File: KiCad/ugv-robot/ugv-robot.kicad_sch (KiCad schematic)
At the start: 2 parts, among them U1 Step Down DC DC

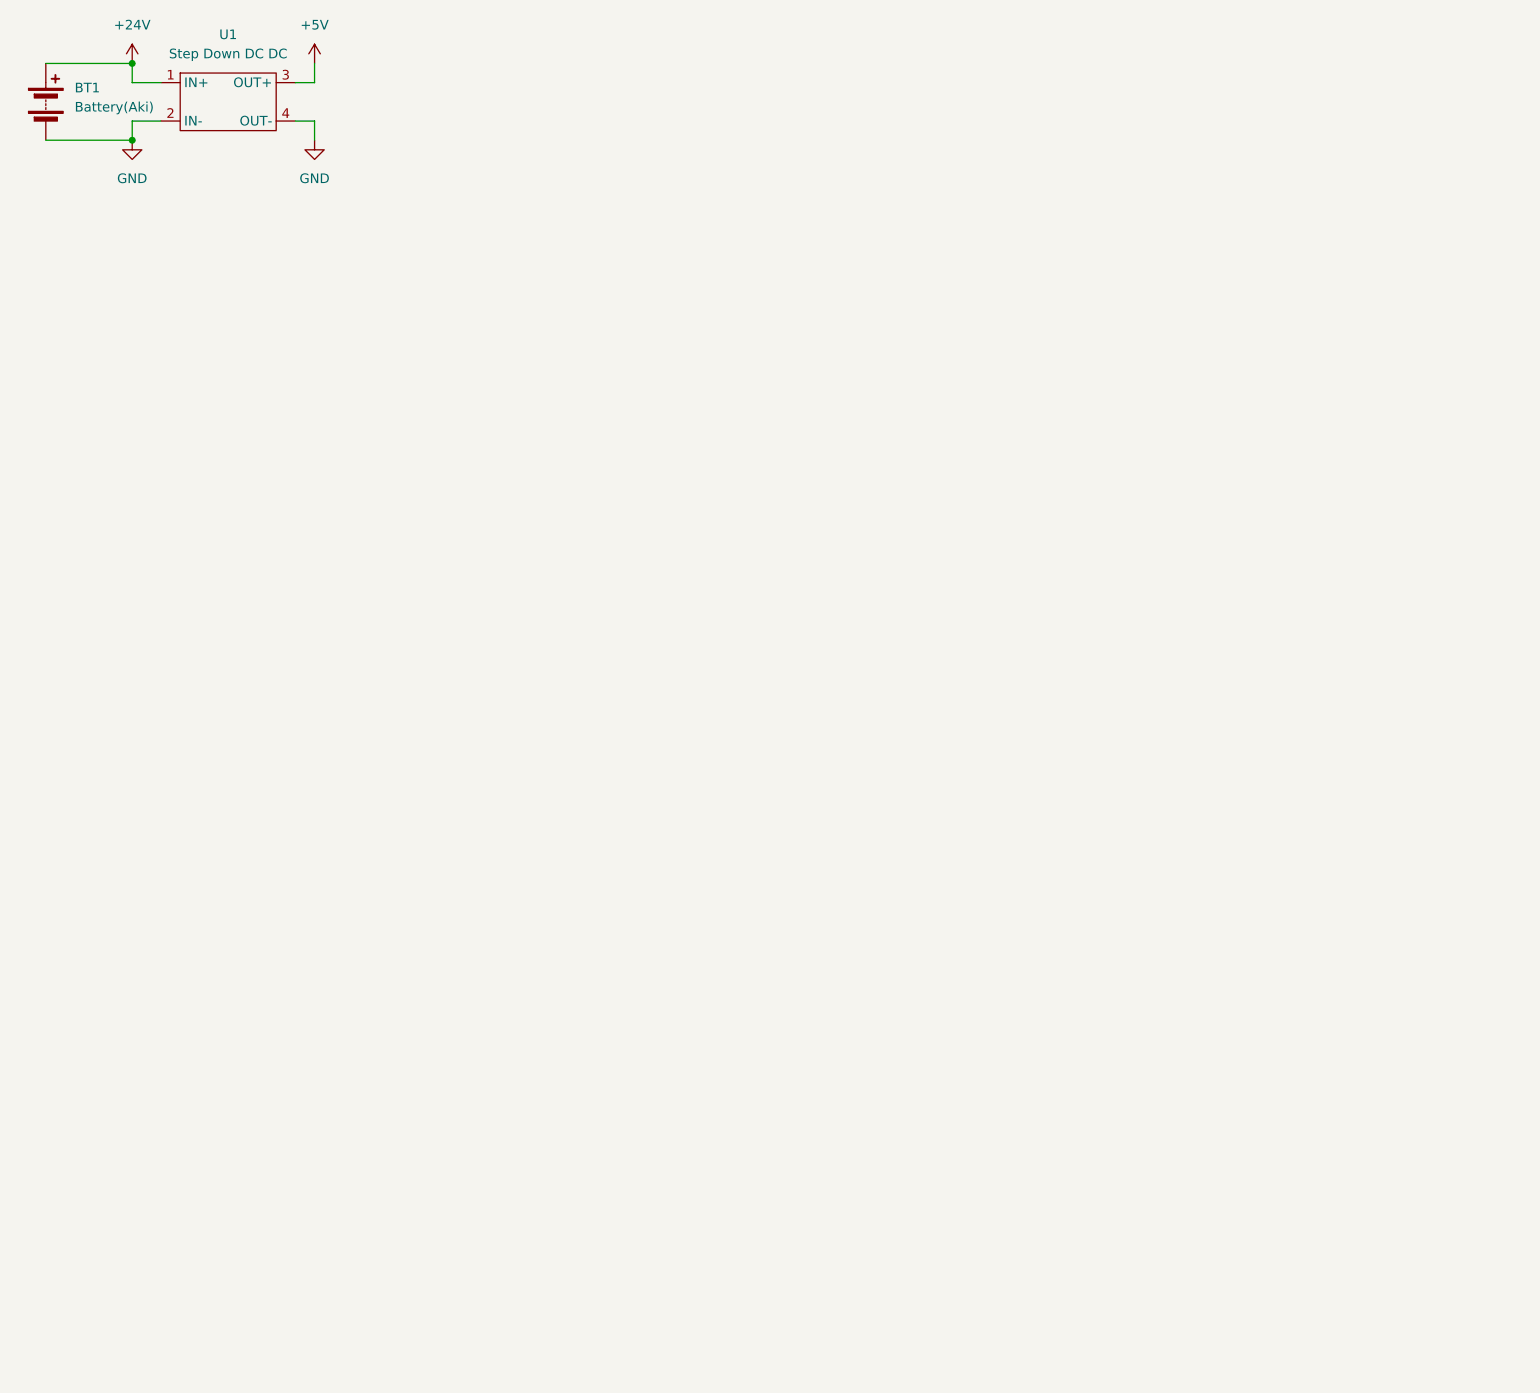
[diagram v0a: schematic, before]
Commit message: KiCad GCS (belum selesai)
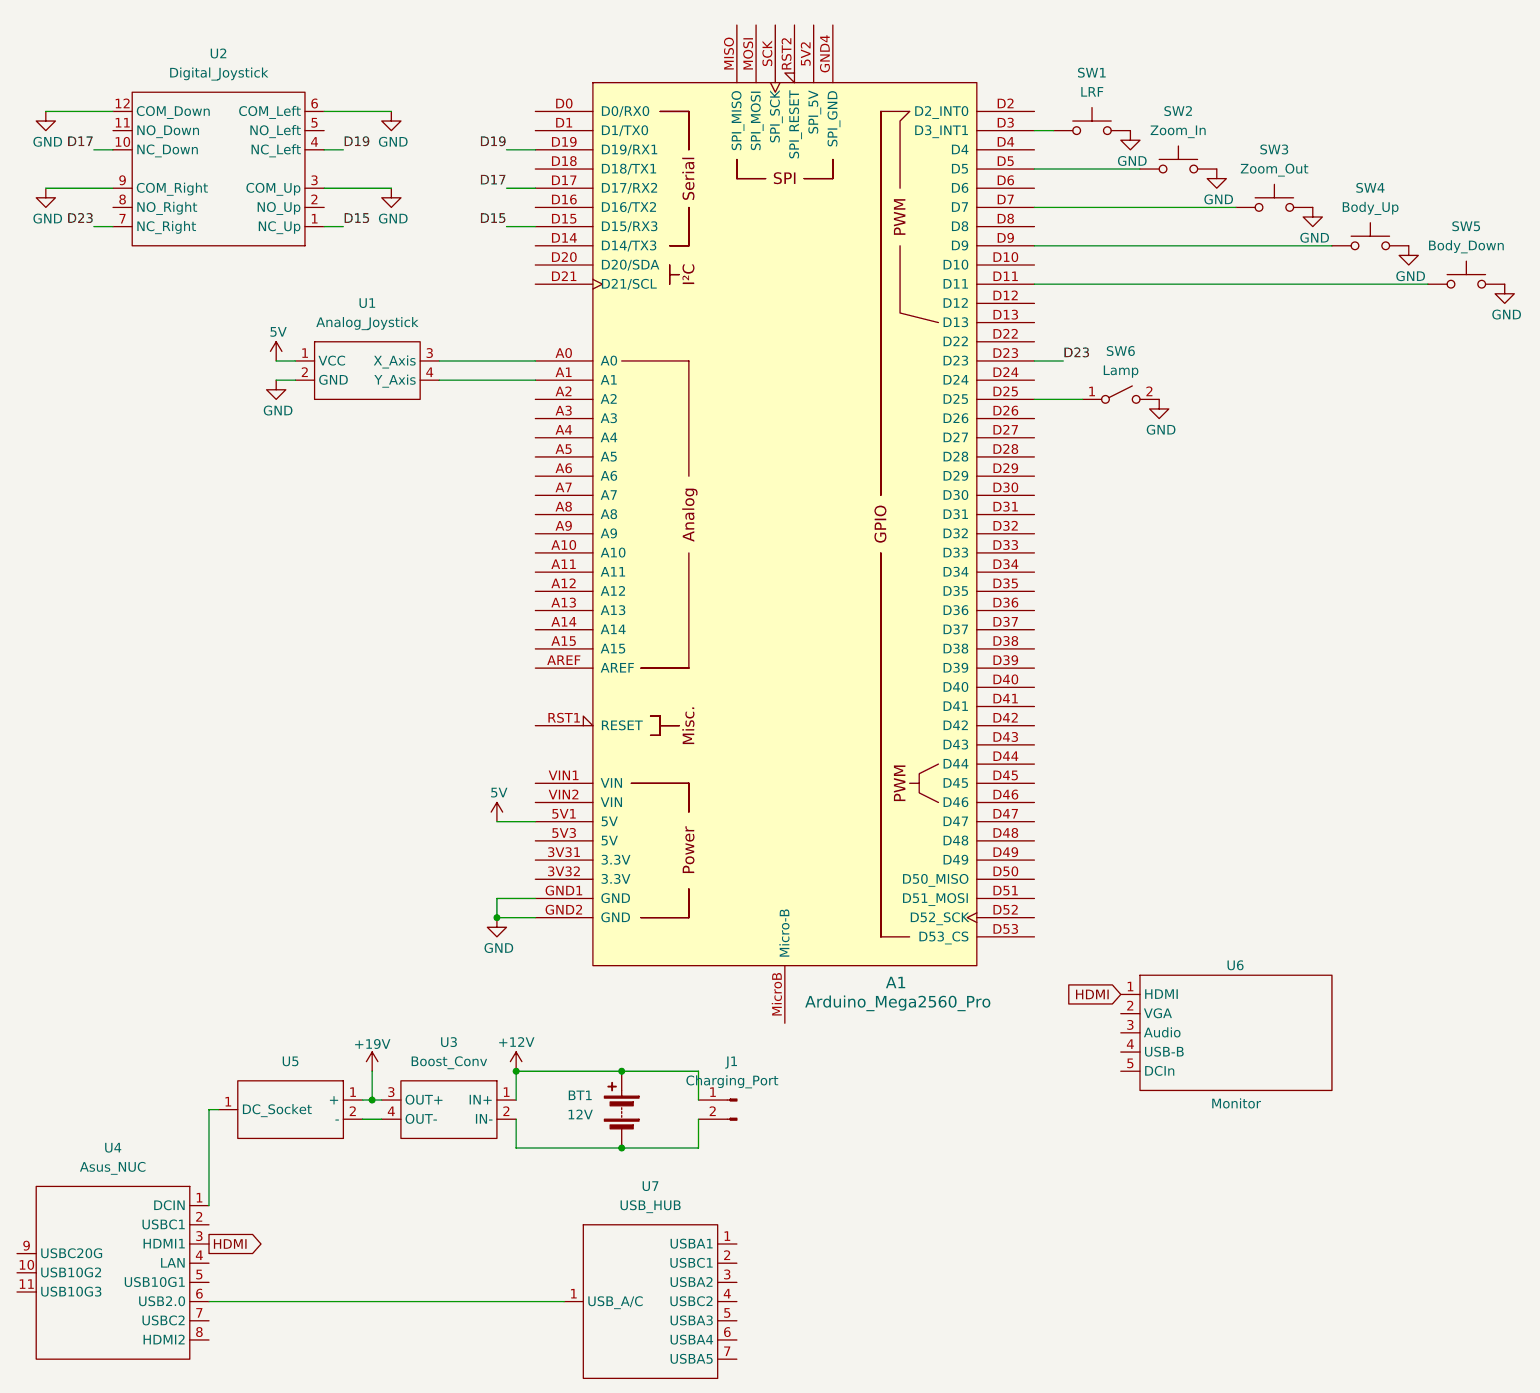
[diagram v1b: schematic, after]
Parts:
- removed U1: Step Down DC DC, symbol bulldozercomp:Step_Module
- added A1: Arduino_Mega2560_Pro, PCM_arduino-library:Clone_Mega2560_Pro_Socket, symbol UGV_Lib:Arduino_Mega2560_Pro
- added J1: Charging_Port, symbol UGV_Lib:Power_Port
- added SW1: LRF, symbol UGV_Lib:SW_Push
- added SW2: Zoom_In, symbol UGV_Lib:SW_Push
- added SW3: Zoom_Out, symbol UGV_Lib:SW_Push
- added SW4: Body_Up, symbol UGV_Lib:SW_Push
- added SW5: Body_Down, symbol UGV_Lib:SW_Push
- added SW6: Lamp, symbol UGV_Lib:SW_Toggle
- added U1: Analog_Joystick, symbol UGV_Lib:Joy_Analog
- added U2: Digital_Joystick, symbol UGV_Lib:Joy_Digital
- added U3: Boost_Conv, symbol UGV_Lib:Boost_Conv
- added U4: Asus_NUC, symbol UGV_Lib:Asus_NUC
- added U5: (no value), symbol UGV_Lib:DCIn_Converter
- added U6: Monitor, symbol UGV_Lib:Monitor
- added U7: USB_HUB, symbol UGV_Lib:USB_HUB
- BT1: value Battery(Aki) -> 12V
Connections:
- net GND: now also A1.GND1 (GND), A1.GND2 (GND), SW1.1, SW2.2, SW3.2, SW4.2, SW5.2, SW6.2 (B), U1.2 (GND), U2.12 (COM_Down), U2.3 (COM_Up), U2.6 (COM_Left), U2.9 (COM_Right); no longer BT1.2 (-)
- net +24V renamed +12V
- net +12V: now also J1.1 (Pin_1), U3.1 (IN+)
- new net: A1.A0, U1.3 (X_Axis)
- new net: A1.A1, U1.4 (Y_Axis)
- new net: A1.D11, SW5.1
- new net: A1.D25, SW6.1 (A)
- new net: A1.D3 (D3_INT1), SW1.2
- new net: A1.D5, SW2.1
- new net: A1.D7, SW3.1
- new net: A1.D9, SW4.1
- new net: U4.1 (DCIN), U5.1 (DC_Socket)
- new net: U4.6 (USB2.0), U7.1 (USBA1)
- new net: BT1.2 (-), J1.2 (Pin_2), U3.2 (IN-)
- new net: U3.4 (OUT-), U5.2 (-)
- new net +19V: U3.3 (OUT+), U5.1 (DC_Socket)
- new net 5V: A1.5V1 (5V), U1.1 (VCC)
- new net D15: A1.D15 (D15/RX3), U2.1 (NC_Up)
- new net D17: A1.D17 (D17/RX2), U2.10 (NC_Down)
- new net D19: A1.D19 (D19/RX1), U2.4 (NC_Left)
- new net D23: A1.D23, U2.7 (NC_Right)
- new net HDMI: U4.3 (HDMI1), U6.1 (HDMI)
